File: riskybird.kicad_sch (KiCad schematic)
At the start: 81 parts, among them J1 USB_B_Micro, J2 Conn_01x02, J3 Conn_01x02, J4 Conn_01x02, J5 Conn_01x02, J6 Conn_01x02, J7 Conn_01x10, J8 Conn_01x10, Q1 SI2302, Q2 SI2302, Q3 SI2302, Q4 SI2302, Q5 DNBT8105-7, Q6 DNBT8105-7, Q7 Q_NMOS_GSD, SW1 SW_SPST, SW2 SW_SPST, SW3 SW_SPST, U1 MCP73831-2-OT, U3 TPS2113A, U4 LP2985-3.0, U5 MPL3115A2, U6 ESP32-C3-WROOM-02, U7 BMI088, U8 FT231XS

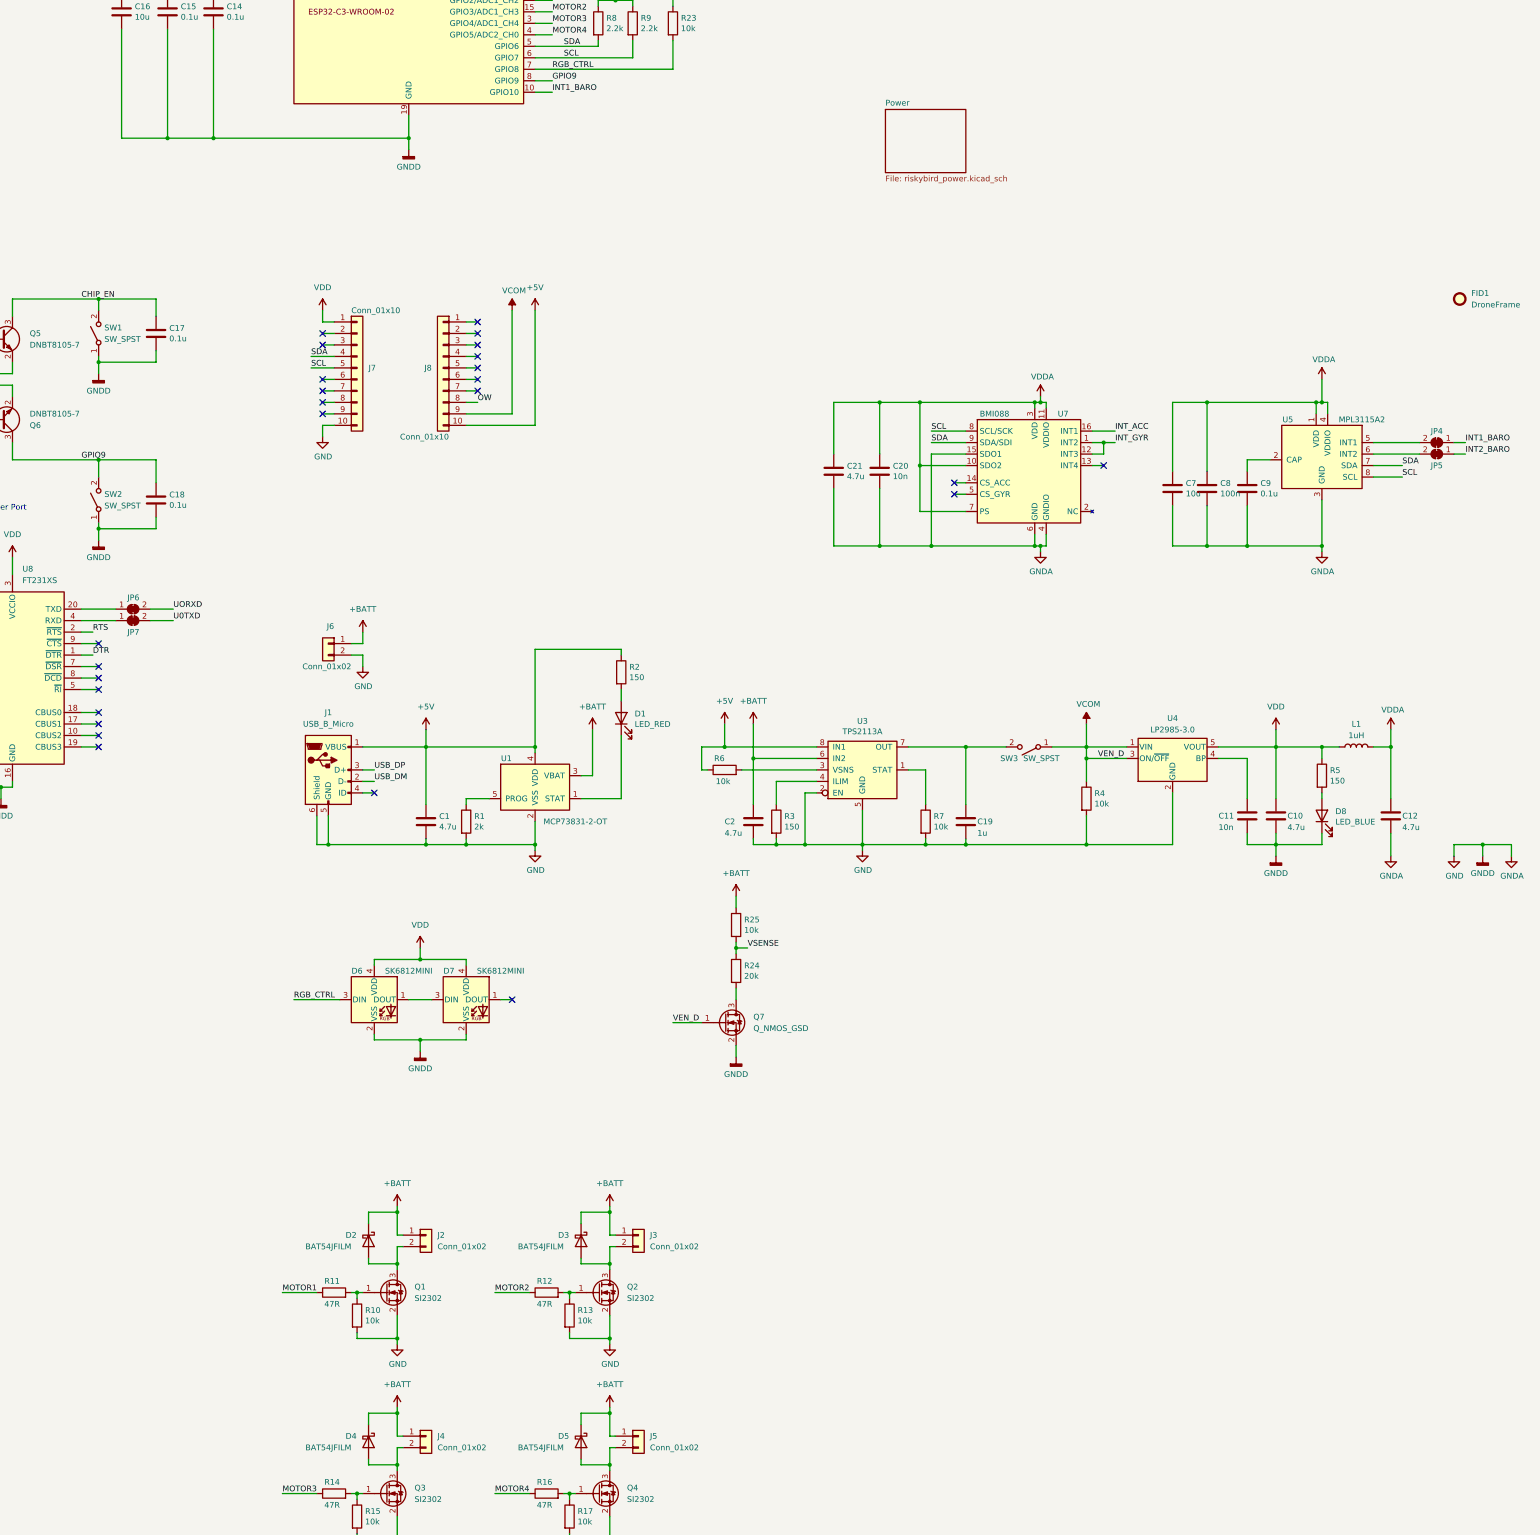
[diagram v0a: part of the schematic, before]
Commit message: almost done routing
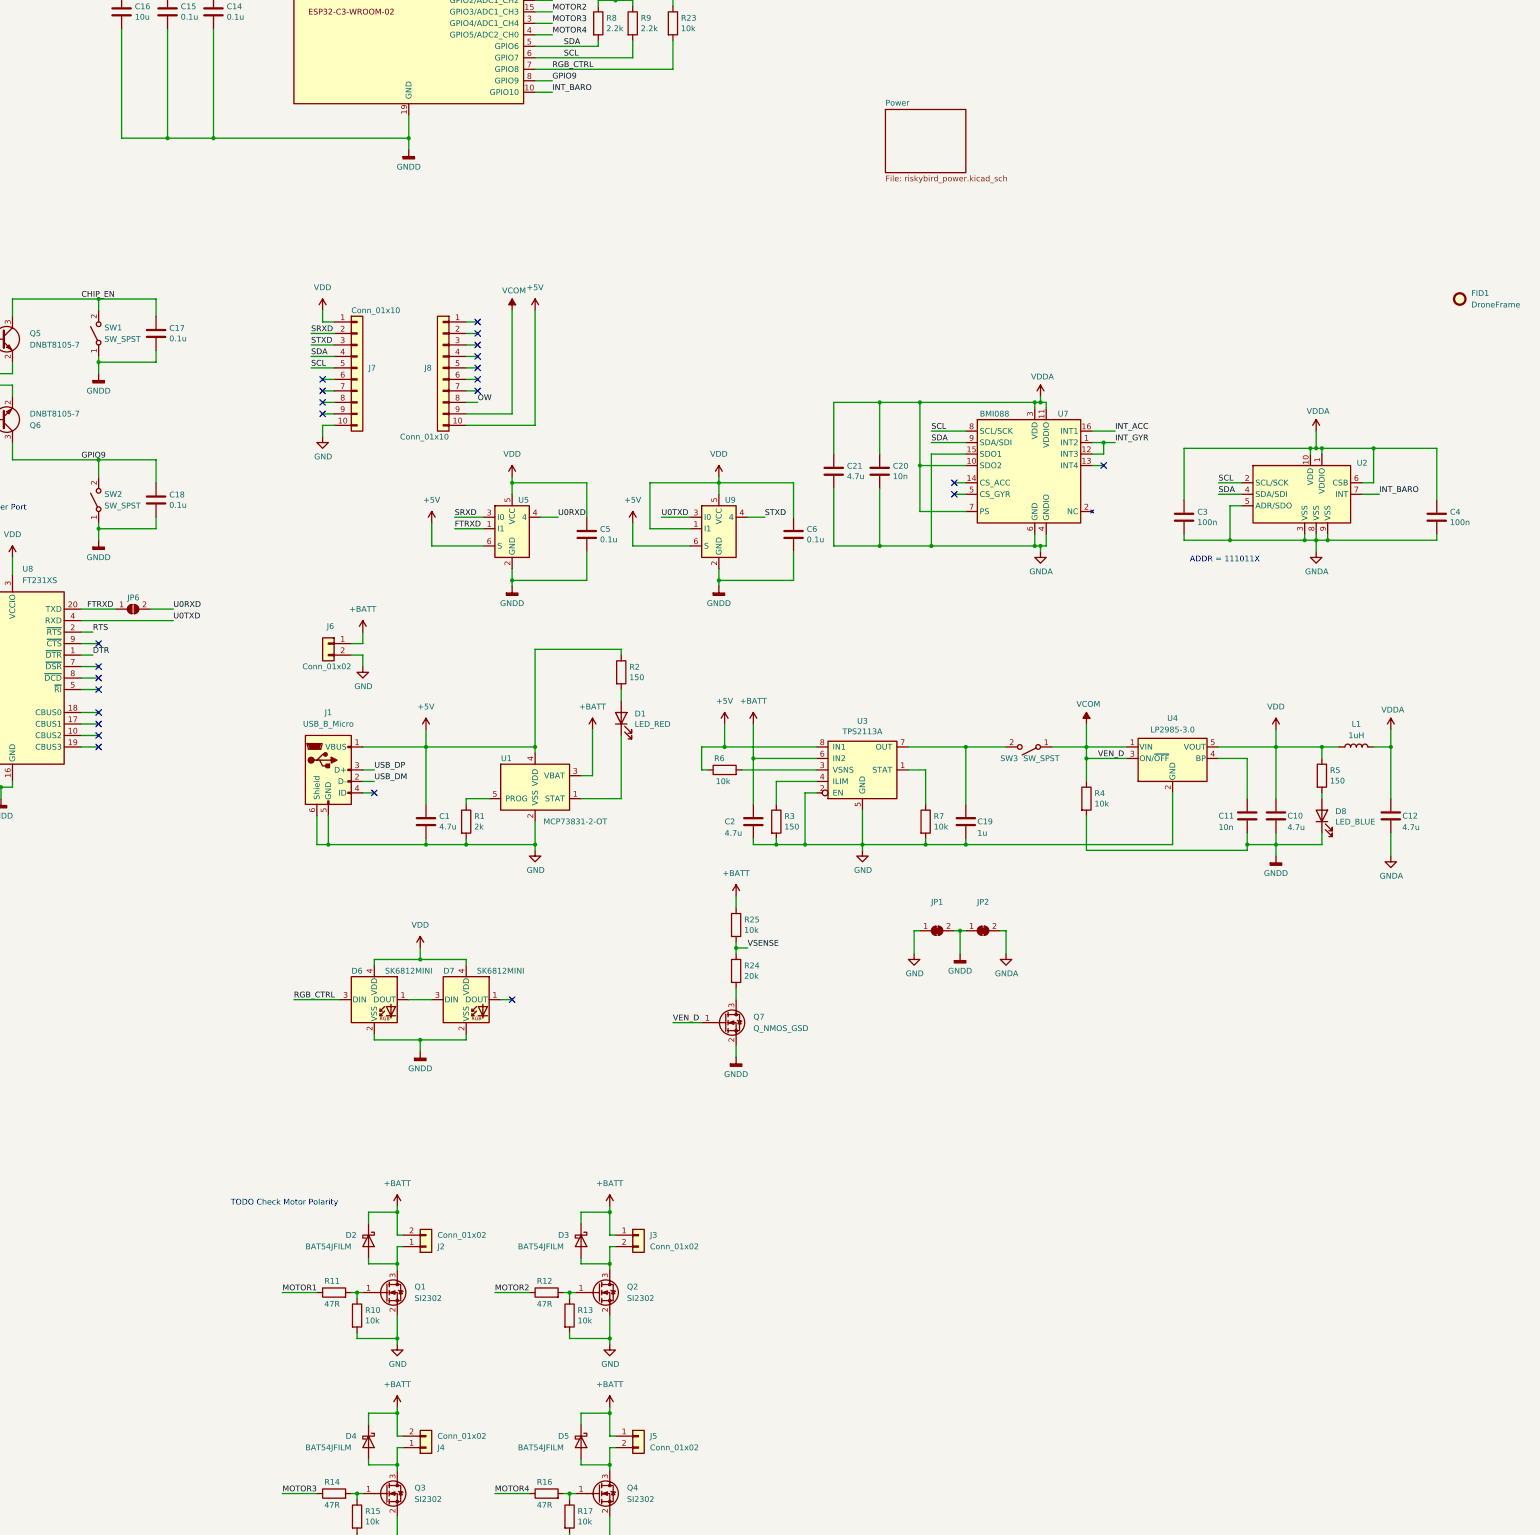
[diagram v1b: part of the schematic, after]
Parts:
- removed C7: 10u, Capacitor_SMD:C_0603_1608Metric_Pad1.08x0.95mm_HandSolder, symbol Device:C
- removed C8: 100n, Capacitor_SMD:C_0603_1608Metric_Pad1.08x0.95mm_HandSolder, symbol Device:C
- removed C9: 0.1u, Capacitor_SMD:C_0603_1608Metric_Pad1.08x0.95mm_HandSolder, symbol Device:C
- removed JP4, JP5, JP7: SolderJumper_2_Bridged, Jumper:SolderJumper-2_P1.3mm_Bridged_Pad1.0x1.5mm, symbol Jumper:SolderJumper_2_Bridged
- removed U5: MPL3115A2, riskybird:MPL3115A2, symbol riskybird-rescue:MPL3115A2-slice
- added C3, C4: 100n, Capacitor_SMD:C_0603_1608Metric_Pad1.08x0.95mm_HandSolder, symbol Device:C
- added C5, C6: 0.1u, Capacitor_SMD:C_0603_1608Metric_Pad1.08x0.95mm_HandSolder, symbol Device:C
- added JP1, JP2: SolderJumper_2_Bridged, Jumper:SolderJumper-2_P1.3mm_Bridged_Pad1.0x1.5mm, symbol Jumper:SolderJumper_2_Bridged
- added U2: ~, riskybird:BMP390_Handsolder, symbol riskybird:BMP390
- added U5, U9: ~, Package_TO_SOT_SMD:SOT-363_SC-70-6, symbol riskybird:74LVC1G157
- JP6: footprint Jumper:SolderJumper-2_P1.3mm_Bridged_Pad1.0x1.5mm -> Jumper:SolderJumper-2_P1.3mm_Open_Pad1.0x1.5mm; symbol Jumper:SolderJumper_2_Bridged -> Jumper:SolderJumper_2_Open
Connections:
- net UORXD is gone; now on net U0RXD: JP6.2 (B)
- net +5V: now also U5.6 (S), U9.6 (S)
- net +BATT: now also J2.2 (Pin_2), J4.2 (Pin_2); no longer J2.1 (Pin_1), J4.1 (Pin_1)
- net GND: now also JP1.1 (A); no longer C10.2, C11.2, C12.2, C13.2, C14.2, C15.2, C16.2, C17.2, C18.2, C20.2, C21.2, D6.2 (VSS), D7.2 (VSS), D8.1 (K), Q7.2 (S), R4.2, SW1.1 (A), SW2.1 (A), U6.19 (GND), U6.9 (GND), U7.15 (SDO1), U7.4 (GNDIO), U7.6 (GND), U8.16 (GND), U8.6 (GND)
- net SCL: now also U2.2 (SCL/SCK)
- net SDA: now also U2.4 (SDA/SDI)
- net U0RXD: now also U5.4
- net U0TXD: now also U8.4 (RXD), U9.3 (I0)
- net VDD: now also C5.1, C6.1, U5.5 (VCC), U9.1 (I1), U9.5 (VCC)
- net VDDA: now also C3.1, C4.1, U2.1 (VDDIO), U2.10 (VDD), U2.6 (CSB)
- net at D4.2 (A), Q3.3 (D): now also J4.1 (Pin_1); no longer J4.2 (Pin_2)
- net at D2.2 (A), Q1.3 (D): now also J2.1 (Pin_1); no longer J2.2 (Pin_2)
- net FTRXD: now reaches JP6.1 (A), U8.20 (TXD)
- net FTRXD: now also U5.1 (I1)
- net SRXD: now reaches J7.2 (Pin_2)
- net SRXD: now also U5.3 (I0)
- net STXD: now reaches J7.3 (Pin_3)
- net STXD: now also U9.4
- net INT1_BARO renamed INT_BARO
- net INT_BARO: now also U2.7 (INT)
- new net GNDA: C12.2, C20.2, C21.2, C3.2, C4.2, JP2.2 (B), U2.3 (VSS), U2.5 (ADR/SDO), U2.8 (VSS), U2.9 (VSS), U7.15 (SDO1), U7.4 (GNDIO), U7.6 (GND)
- new net GNDD: C10.2, C11.2, C13.2, C14.2, C15.2, C16.2, C17.2, C18.2, C5.2, C6.2, D6.2 (VSS), D7.2 (VSS), D8.1 (K), JP1.2 (B), JP2.1 (A), Q7.2 (S), R4.2, SW1.1 (A), SW2.1 (A), U5.2 (GND), U6.19 (GND), U6.9 (GND), U8.16 (GND), U8.6 (GND), U9.2 (GND)
- no-connect marks 27 -> 25
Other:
- note added: "ADDR = 111011X"
- note added: "TODO Check Motor Polarity"
